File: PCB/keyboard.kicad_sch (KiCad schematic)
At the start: 153 parts, among them J1 JST SH 4-pin, SW1 SW_Push, U1 ATmega32U4-A, U2 SRV05-4, Y1 16MHz

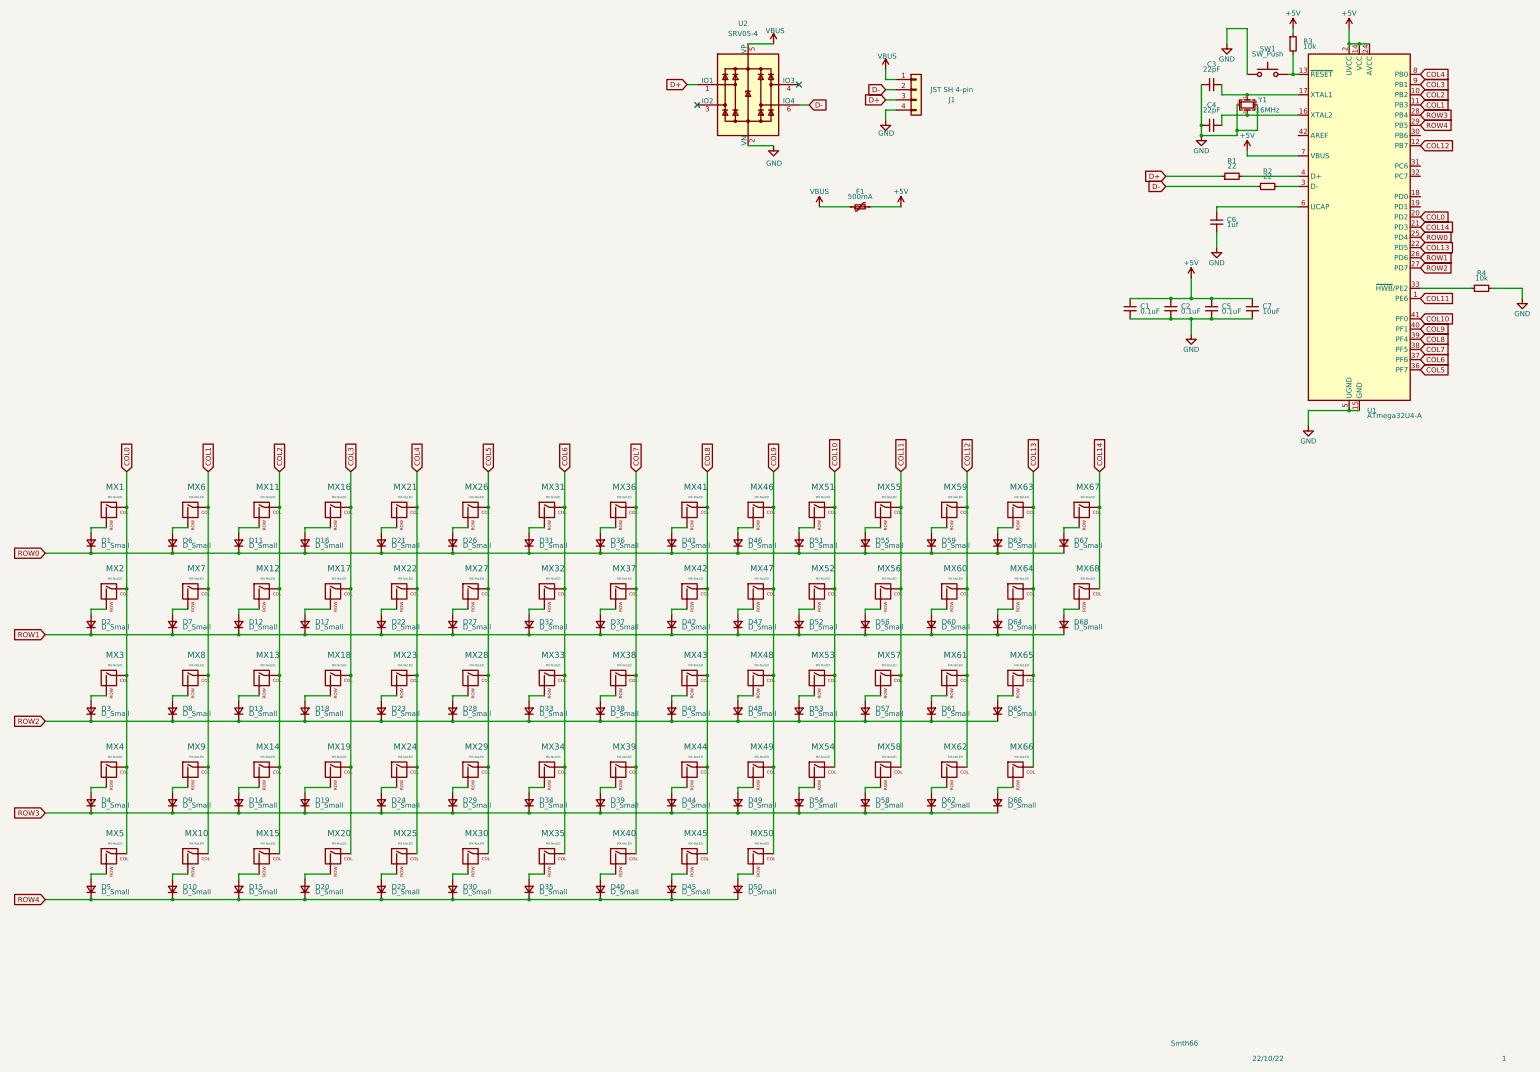
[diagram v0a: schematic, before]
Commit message: all new pretty wiring
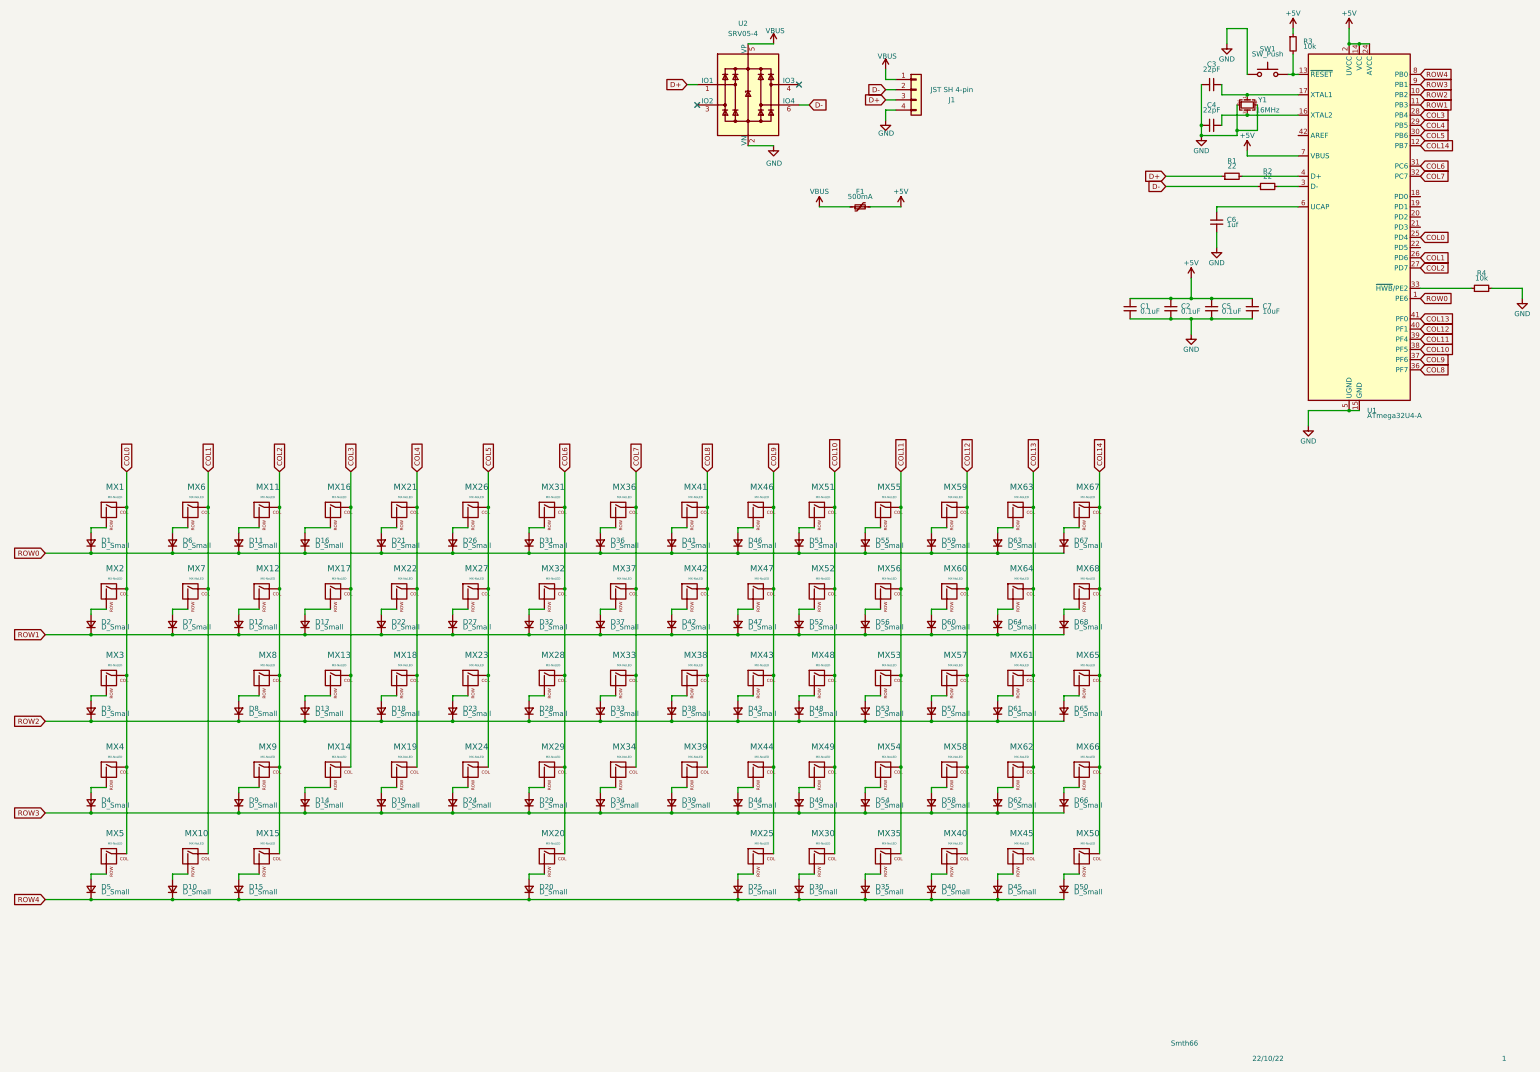
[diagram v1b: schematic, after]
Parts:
- removed D20, D25, D8, D9: D_Small, Diode_SMD:D_SOD-123, symbol Device:D_Small
- added D35, D50, D65, D66: D_Small, Diode_SMD:D_SOD-123, symbol Device:D_Small
- renumbered D18 to D13, D19 to D14, D23 to D18, D24 to D19, D35 to D20, D28 to D23, D29 to D24, D50 to D25, D33 to D28, D34 to D29, D38 to D33, D39 to D34, D43 to D38, D44 to D39, D48 to D43, D49 to D44, D53 to D48, D54 to D49, D57 to D53, D58 to D54, D61 to D57, D62 to D58, D65 to D61, D66 to D62, D13 to D8, D14 to D9
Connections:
- net COL0: now also U1.25 (PD4); no longer U1.20 (PD2)
- net COL1: now also U1.26 (PD6); no longer MX8.1 (COL), MX9.1 (COL), U1.11 (PB3)
- net COL10: now also MX30.1 (COL), MX48.1 (COL), MX49.1 (COL), U1.38 (PF5); no longer MX53.1 (COL), MX54.1 (COL), U1.41 (PF0)
- net COL11: now also MX35.1 (COL), MX53.1 (COL), MX54.1 (COL), U1.39 (PF4); no longer MX57.1 (COL), MX58.1 (COL), U1.1 (PE6)
- net COL12: now also MX40.1 (COL), MX57.1 (COL), MX58.1 (COL), U1.40 (PF1); no longer MX61.1 (COL), MX62.1 (COL), U1.12 (PB7)
- net COL13: now also MX45.1 (COL), MX61.1 (COL), MX62.1 (COL), U1.41 (PF0); no longer MX65.1 (COL), MX66.1 (COL), U1.22 (PD5)
- net COL14: now also MX50.1 (COL), MX65.1 (COL), MX66.1 (COL), U1.12 (PB7); no longer U1.21 (PD3)
- net COL2: now also MX8.1 (COL), MX9.1 (COL), U1.27 (PD7); no longer MX13.1 (COL), MX14.1 (COL), U1.10 (PB2)
- net COL3: now also MX13.1 (COL), MX14.1 (COL), U1.28 (PB4); no longer MX18.1 (COL), MX19.1 (COL), MX20.1 (COL), U1.9 (PB1)
- net COL4: now also MX18.1 (COL), MX19.1 (COL), U1.29 (PB5); no longer MX23.1 (COL), MX24.1 (COL), MX25.1 (COL), U1.8 (PB0)
- net COL5: now also MX23.1 (COL), MX24.1 (COL), U1.30 (PB6); no longer MX28.1 (COL), MX29.1 (COL), MX30.1 (COL), U1.36 (PF7)
- net COL6: now also MX20.1 (COL), MX28.1 (COL), MX29.1 (COL), U1.31 (PC6); no longer MX33.1 (COL), MX34.1 (COL), MX35.1 (COL), U1.37 (PF6)
- net COL7: now also MX33.1 (COL), MX34.1 (COL), U1.32 (PC7); no longer MX38.1 (COL), MX39.1 (COL), MX40.1 (COL), U1.38 (PF5)
- net COL8: now also MX38.1 (COL), MX39.1 (COL), U1.36 (PF7); no longer MX43.1 (COL), MX44.1 (COL), MX45.1 (COL), U1.39 (PF4)
- net COL9: now also MX25.1 (COL), MX43.1 (COL), MX44.1 (COL), U1.37 (PF6); no longer MX48.1 (COL), MX49.1 (COL), MX50.1 (COL), U1.40 (PF1)
- net ROW0: now also U1.1 (PE6); no longer U1.25 (PD4)
- net ROW1: now also U1.11 (PB3); no longer U1.26 (PD6)
- net ROW2: now also U1.10 (PB2), D65.1 (K); no longer U1.27 (PD7)
- net ROW3: now also U1.9 (PB1), D66.1 (K); no longer U1.28 (PB4)
- net ROW4: now also U1.8 (PB0), D35.1 (K), D50.1 (K); no longer U1.29 (PB5)
- net at MX34.2 (ROW): now also D34.2 (A); no longer D29.2 (A)
- net at MX48.2 (ROW): now also D48.2 (A); no longer D43.2 (A)
- net at MX20.2 (ROW): now also D20.2 (A)
- net at MX35.2 (ROW): now also D35.2 (A); no longer D20.2 (A)
- net at MX39.2 (ROW): now also D39.2 (A); no longer D34.2 (A)
- net at MX61.2 (ROW): now also D61.2 (A); no longer D57.2 (A)
- net at D8.2 (A): now also MX8.2 (ROW); no longer MX13.2 (ROW)
- net at D54.2 (A): now also MX54.2 (ROW); no longer MX58.2 (ROW)
- net at MX57.2 (ROW): now also D57.2 (A); no longer D53.2 (A)
- net at D58.2 (A): now also MX58.2 (ROW); no longer MX62.2 (ROW)
- net at D13.2 (A): now also MX13.2 (ROW); no longer MX18.2 (ROW)
- net at MX65.2 (ROW): now also D65.2 (A); no longer D61.2 (A)
- net at MX49.2 (ROW): now also D49.2 (A); no longer D44.2 (A)
- net at MX9.2 (ROW): now also D9.2 (A)
- net at MX14.2 (ROW): now also D14.2 (A); no longer D9.2 (A)
- net at MX33.2 (ROW): now also D33.2 (A); no longer D28.2 (A)
- net at MX38.2 (ROW): now also D38.2 (A); no longer D33.2 (A)
- net at MX23.2 (ROW): now also D23.2 (A); no longer D18.2 (A)
- net at MX25.2 (ROW): now also D25.2 (A)
- net at MX19.2 (ROW): now also D19.2 (A); no longer D14.2 (A)
- net at MX28.2 (ROW): now also D28.2 (A); no longer D23.2 (A)
- net at MX50.2 (ROW): now also D50.2 (A); no longer D25.2 (A)
- net at MX24.2 (ROW): now also D24.2 (A); no longer D19.2 (A)
- net at MX43.2 (ROW): now also D43.2 (A); no longer D38.2 (A)
- net at D62.2 (A): now also MX62.2 (ROW); no longer MX66.2 (ROW)
- net at MX44.2 (ROW): now also D44.2 (A); no longer D39.2 (A)
- net at MX53.2 (ROW): now also D53.2 (A); no longer D48.2 (A)
- net at MX29.2 (ROW): now also D29.2 (A); no longer D24.2 (A)
- new net: D18.2 (A), MX18.2 (ROW)
- new net: D66.2 (A), MX66.2 (ROW)
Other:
- moved on the sheet: MX13, MX14, MX18, MX19, MX20, MX23, MX24, MX25, MX28, MX29, MX30, MX33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

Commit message: Redid wiring again
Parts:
- U2: footprint Package_TO_SOT_SMD:SOT-23-6 -> marbastlib-various:SOT-23-6-routable
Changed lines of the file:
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@@
       (effects (font (size 1.27 1.27)))
     )
-    (property "Footprint" "Package_TO_SOT_SMD:SOT-23-6" (id 2) (at 223.52 50.8 0)
+    (property "Footprint" "marbastlib-various:SOT-23-6-routable" (id 2) (at 223.52 50.8 0)
       (effects (font (size 1.27 1.27)) hide)
     )
@@
     )
     (path "/ef12052d-f84d-46d8-a991-3451abdfdbc0"
-      (reference "U2") (unit 1) (value "SRV05-4") (footprint "Package_TO_SOT_SMD:SOT-23-6")
+      (reference "U2") (unit 1) (value "SRV05-4") (footprint "marbastlib-various:SOT-23-6-routable")
     )
     (path "/554c564d-e286-4b2b-aa94-325d745117a1"
